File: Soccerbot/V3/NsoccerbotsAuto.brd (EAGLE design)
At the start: 149.8 x 101.3 mm, 69 parts, among them CN2 1X4-CLEANBIG, IC1 LM340S-05, IC2 TB6612FNG, IC4 TB6612FNG, J3 1X5, J4 1X5, Q1 AOD417, SW2 SPST_TACT-EVQQ2, U1 PCA9685, X1 NXT-SOCKET, X2 NXT-SOCKET, X3 NXT-SOCKET, X4 NXT-SOCKET

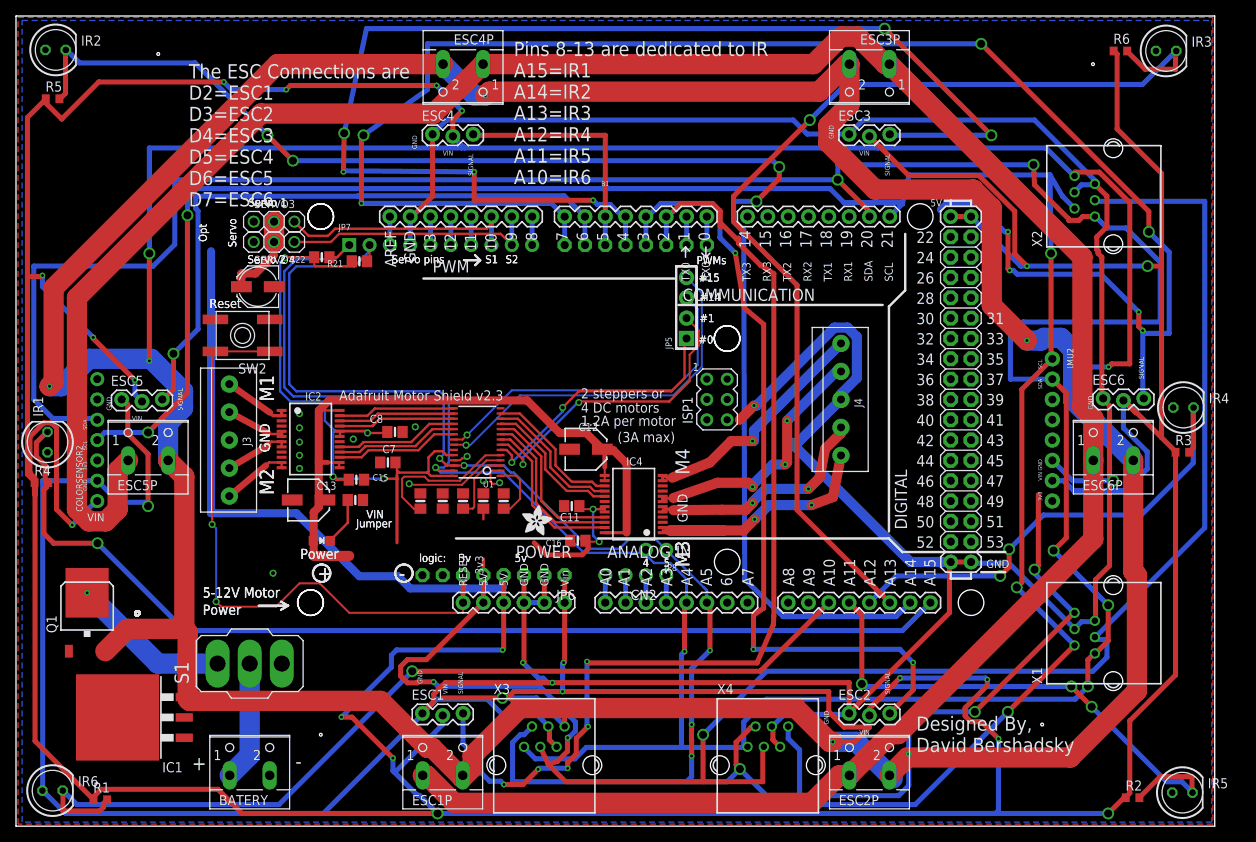
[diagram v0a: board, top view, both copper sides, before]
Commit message: S
S
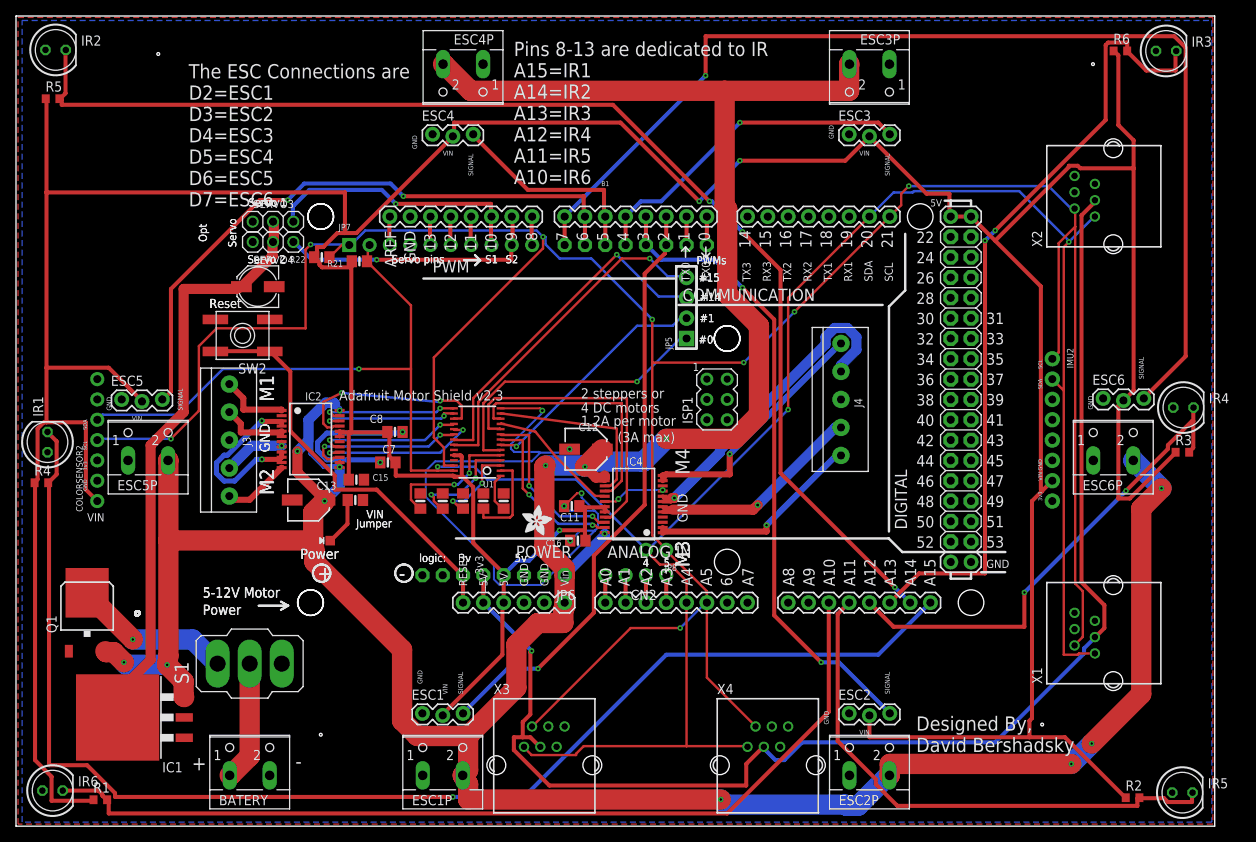
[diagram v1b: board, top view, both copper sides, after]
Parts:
- moved SERVO3 0.13 mm to (42.3, 74.3)
- moved SERVO4 0.13 mm to (42.3, 71.8)
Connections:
- new net A0A: B1.A0, CN2.4
- new net A1A: B1.A1, CN2.3
- new net A2A: B1.A2, CN2.2
- new net A3A: B1.A3, CN2.1
- net 5.5V: no longer C14.+
- net A0: no longer B1.A0, CN2.4
- net A1: no longer B1.A1, CN2.3
- net A2: no longer B1.A2, CN2.2
- net A3: no longer B1.A3, CN2.1
- net SERVO5V: now also C14.+
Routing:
- net GND: track 846.5 -> 134.7 mm, vias 15 -> 11
- net BAT+: track 878.3 -> 449.0 mm, vias 13 -> 14
- net 5.5V: track 813.2 -> 581.4 mm, vias 24 -> 3
- net SDA: track 473.0 -> 310.2 mm, vias 7 -> 4
- net D4: track 157.9 -> 42.1 mm, vias 6 -> 1
- net SCL: track 442.7 -> 356.9 mm, vias 11 -> 8
- net D7: track 217.2 -> 140.0 mm, vias 8 -> 1
- net SERVO5V: track 2.54 -> 74.2 mm
- net D2: track 128.4 -> 74.9 mm, vias 5 -> 1
- net 3.3V: track 224.6 -> 171.3 mm, vias 3 -> 1
- net A15: track 131.8 -> 164.7 mm
- net A13: track 131.1 -> 99.2 mm, vias 1 -> 2
- net A14: track 181.4 -> 154.1 mm, vias 4 -> 3
- net RESET: track 77.0 -> 51.4 mm, vias 2 -> 0
- net D3: track 99.5 -> 80.0 mm, vias 3 -> 2
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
